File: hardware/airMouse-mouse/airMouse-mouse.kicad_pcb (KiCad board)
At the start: 2 copper layers, 50 x 23 mm, 18 parts, among them J1 DS1020-07-10VBT1A-R, SW1 KEY, SW2 KEY, SW3 KEY, SW4 KEY, SW5 KEY, SW6 KEY, SW7 KEY, SW8 KEY

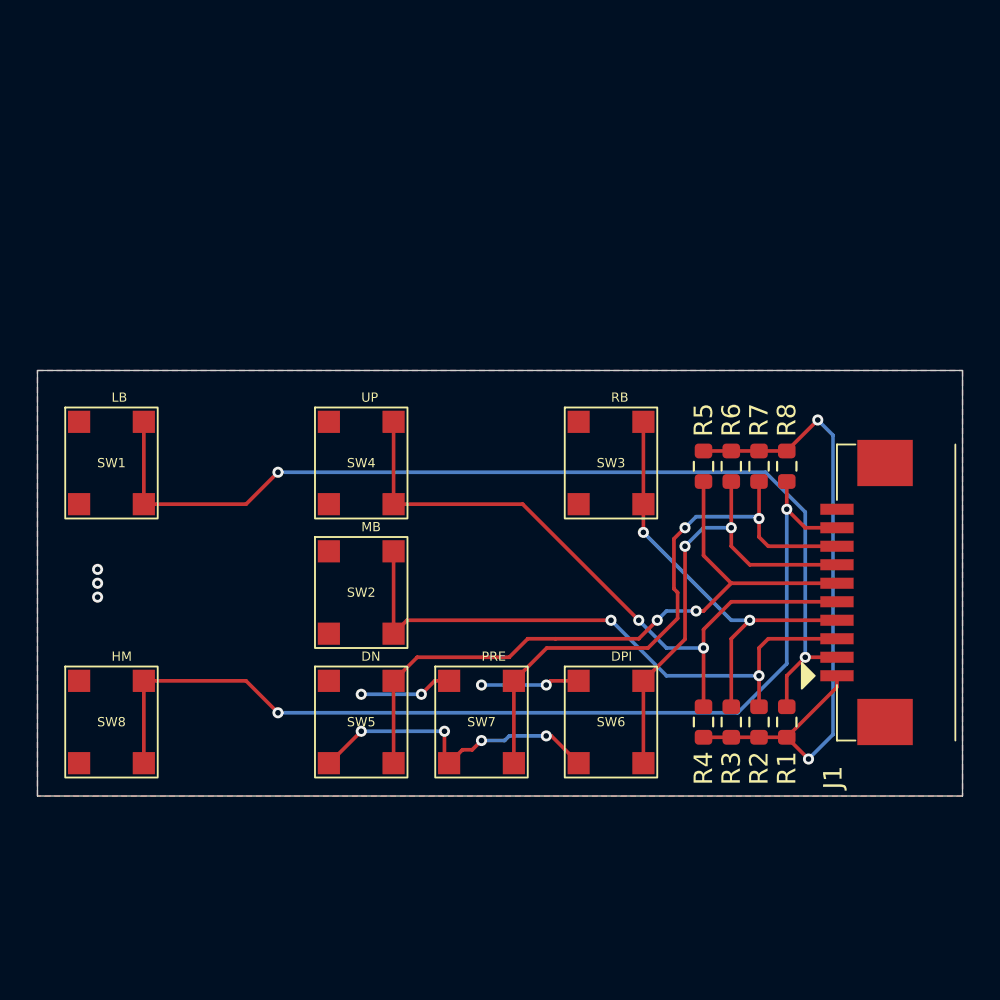
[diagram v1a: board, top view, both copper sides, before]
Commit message: mini2 frame
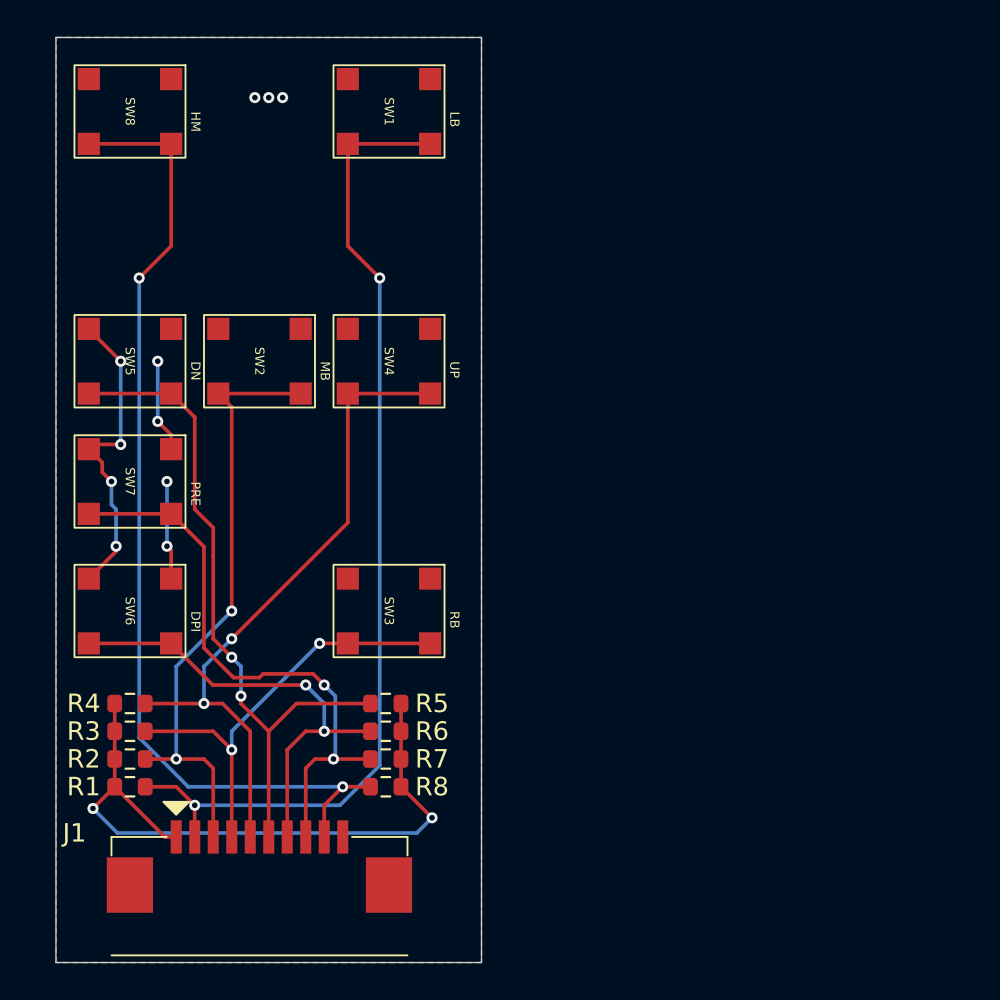
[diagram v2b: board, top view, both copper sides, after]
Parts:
- moved R1 35.7 mm to (121.0, 90.5), turned to 0 degrees
- moved R2 34.1 mm to (121.0, 89.0), turned to 0 degrees
- moved J1 33.9 mm to (128.0, 93.2), turned to 0 degrees
- moved SW8 33.0 mm to (121.0, 54.0), turned to -90 degrees
- moved R3 32.5 mm to (121.0, 87.5), turned to 0 degrees
- moved R4 31.0 mm to (121.0, 86.0), turned to 0 degrees
- moved R8 27.7 mm to (134.8, 90.5), turned to 180 degrees
- moved SW6 26.7 mm to (121.0, 81.0), turned to -90 degrees
- moved R7 25.6 mm to (134.8, 89.0), turned to 180 degrees
- moved SW1 24.2 mm to (135.0, 54.0), turned to -90 degrees
- moved R6 23.5 mm to (134.8, 87.5), turned to 180 degrees
- moved SW5 23.2 mm to (121.0, 67.5), turned to -90 degrees
- moved SW7 23.0 mm to (121.0, 74.0), turned to -90 degrees
- moved R5 21.4 mm to (134.8, 86.0), turned to 180 degrees
- moved SW3 14.4 mm to (135.0, 81.0), turned to -90 degrees
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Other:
- board size 50 x 23 mm -> 23 x 50 mm
